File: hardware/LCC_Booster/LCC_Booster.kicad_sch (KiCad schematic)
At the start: 16 parts, among them J1 A00-216-262-450, J2 54-00166, J3 Screw_Terminal_01x08, SW1 SW_Push, U1 ACPL-214-500E, U2 ACPL-214-500E

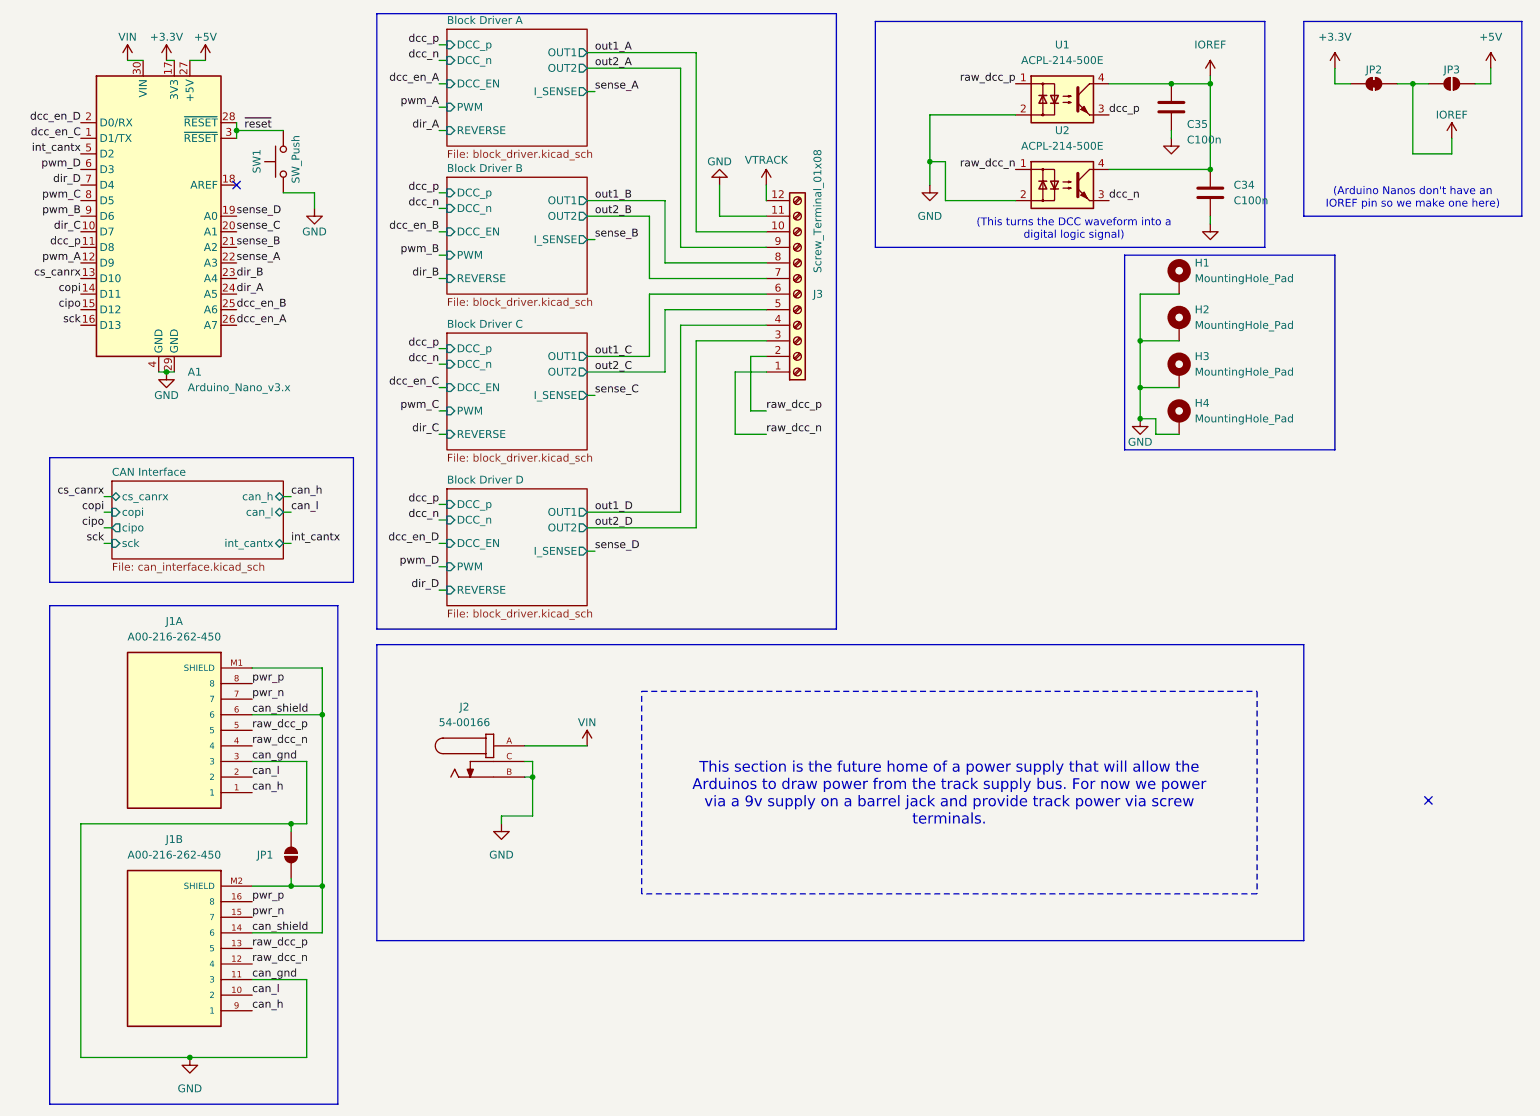
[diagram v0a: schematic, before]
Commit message: Update Schematic
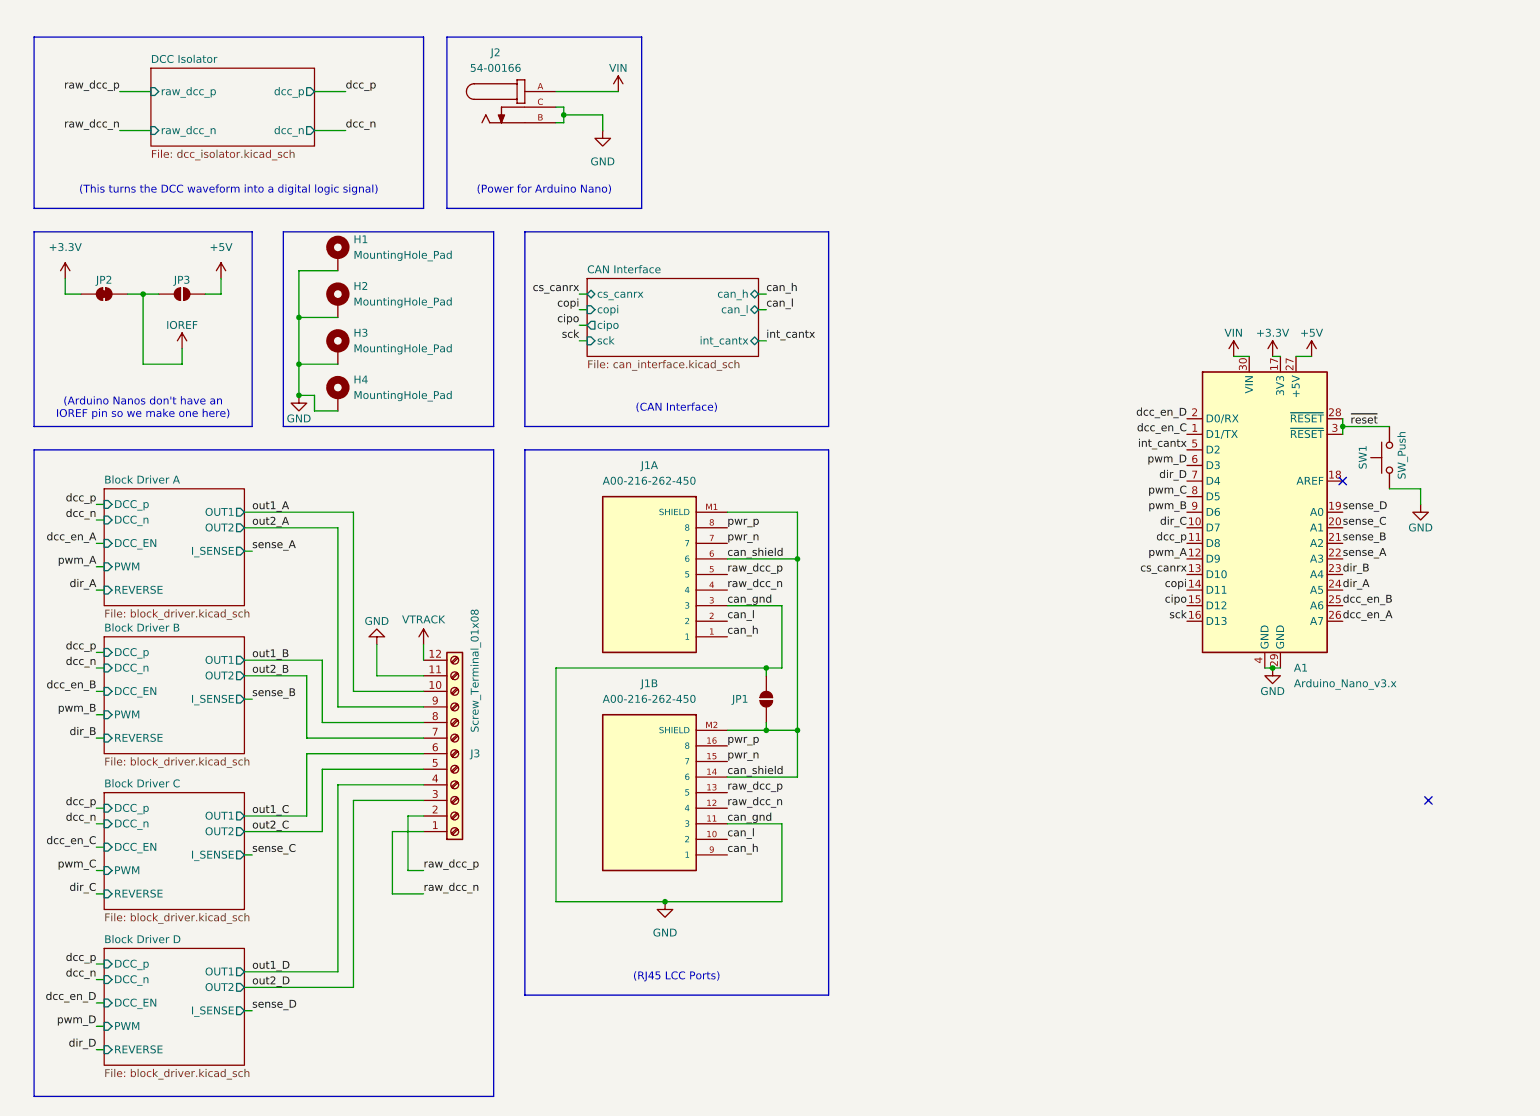
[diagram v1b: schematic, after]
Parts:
- removed C34, C35: C100n, Capacitor_SMD:C_0402_1005Metric_Pad0.74x0.62mm_HandSolder, symbol Device:C
- removed U1, U2: ACPL-214-500E, Package_SO:SOP-4_4.4x2.6mm_P1.27mm, symbol Isolator:ACPL-214-500E
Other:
- added sheet DCC Isolator (dcc_isolator.kicad_sch)
- moved on the sheet: A1, H1, H2, H3, H4, J1A, J1B, J2, J3, JP1, JP2, JP3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
